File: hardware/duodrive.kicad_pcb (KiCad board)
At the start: 2 copper layers, 49 x 75 mm, 113 parts, among them J2 Conn_02x08_Odd_Even, J3 SWD, J4 CAN_IN, J5 CAN_OUT, J6 POWER, J7 ENCODER1, J8 ENCODER2, Q1 AOD4184, Q2 AOD4184, Q3 AOD4184, Q4 AOD4184, Q5 AOD4184, Q6 AOD4184, Q7 AOD4184, Q8 AOD4184, U1 TCAN1044V, U10 MIC5219-3.3YM5, U2 IR2011, U3 TPS62173DSG, U4 STM32G431RBTx, U5 IR2011, U6 IR2011, U7 IR2011, U8 TPS62933, Y1 Resonator

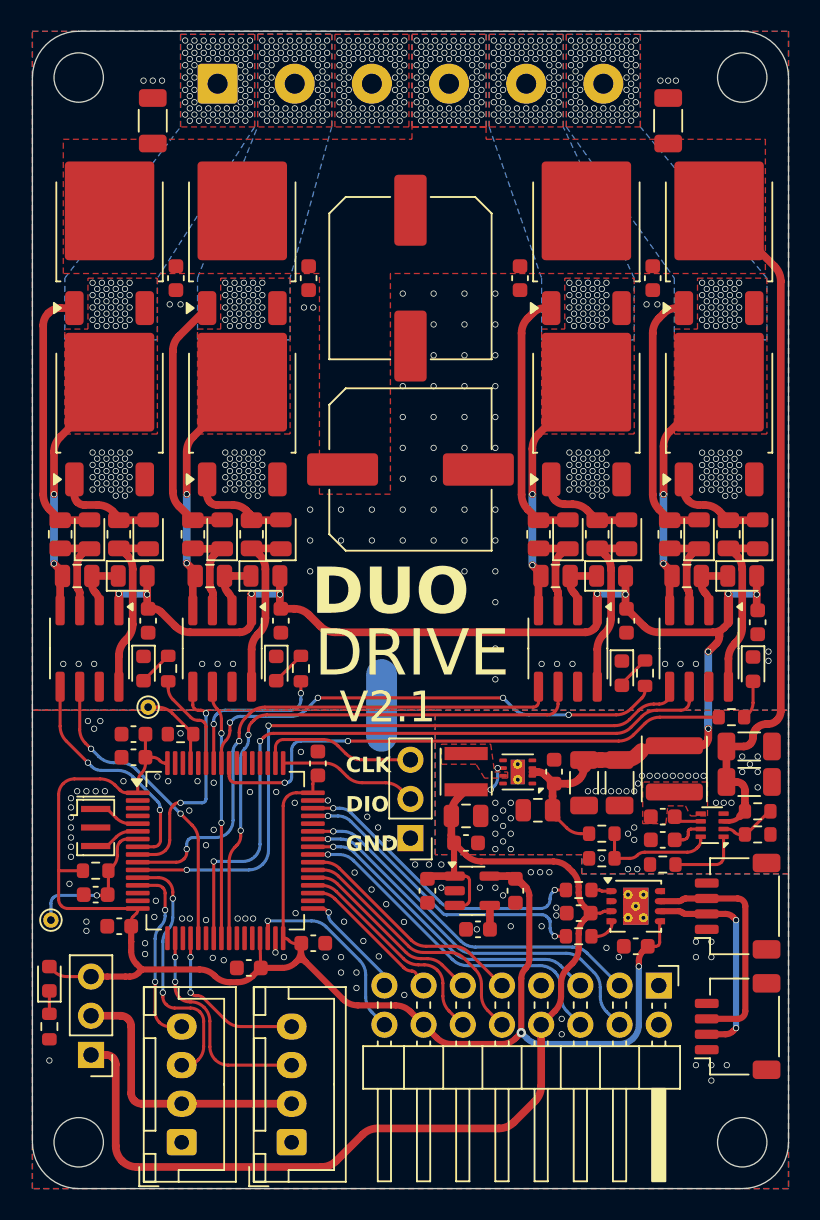
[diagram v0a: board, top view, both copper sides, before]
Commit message: polishing
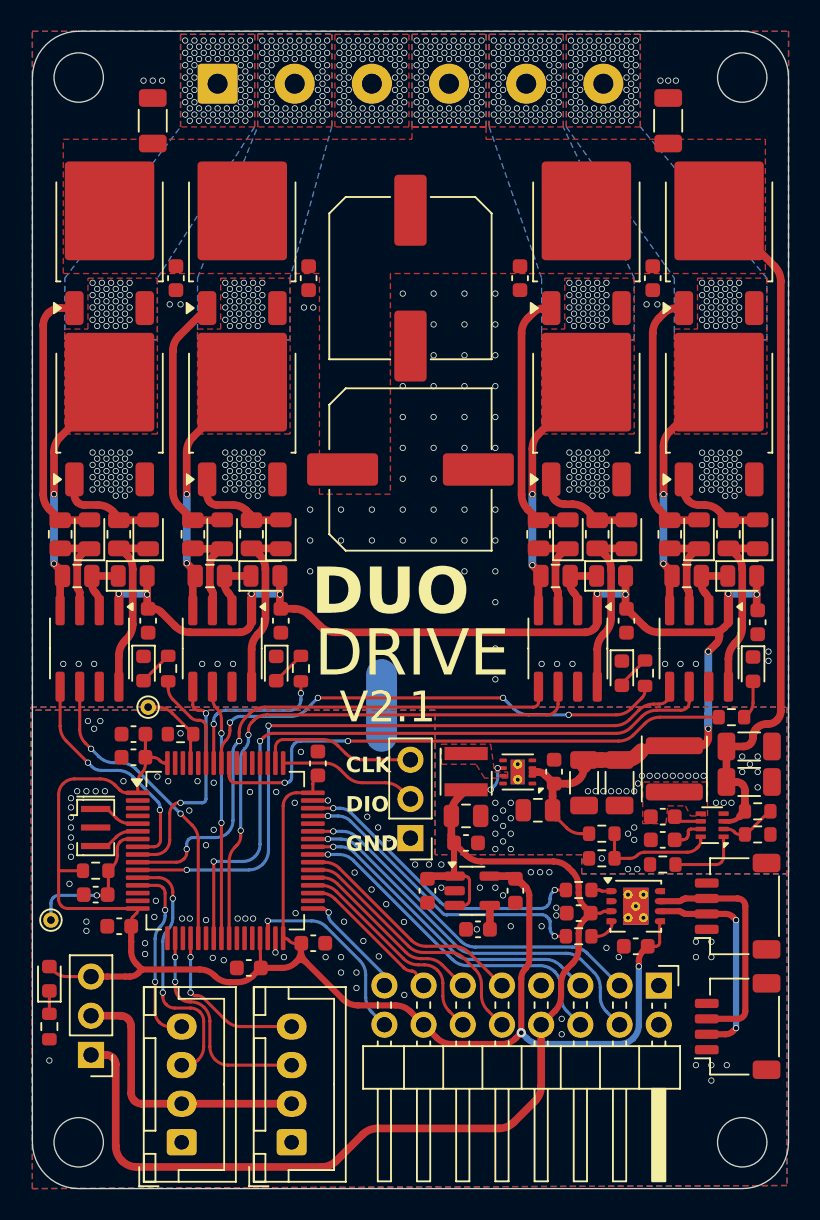
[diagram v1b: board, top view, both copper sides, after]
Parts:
- R4: value 11.8K -> 115K
- R6: value 1K -> 10K
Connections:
- U4 pad 34: CANSET -> unconnected-(U4-PB12-Pad34)
